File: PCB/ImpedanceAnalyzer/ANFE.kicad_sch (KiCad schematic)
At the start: 61 parts, among them U1 LTC2311, U10 OPA350, U11 OPA350, U2 LTC2311, U3 REF02Z, U4 LD1117S25-TR, U5 LD1117S50-TR, U7 LT1819, U9 OPA350

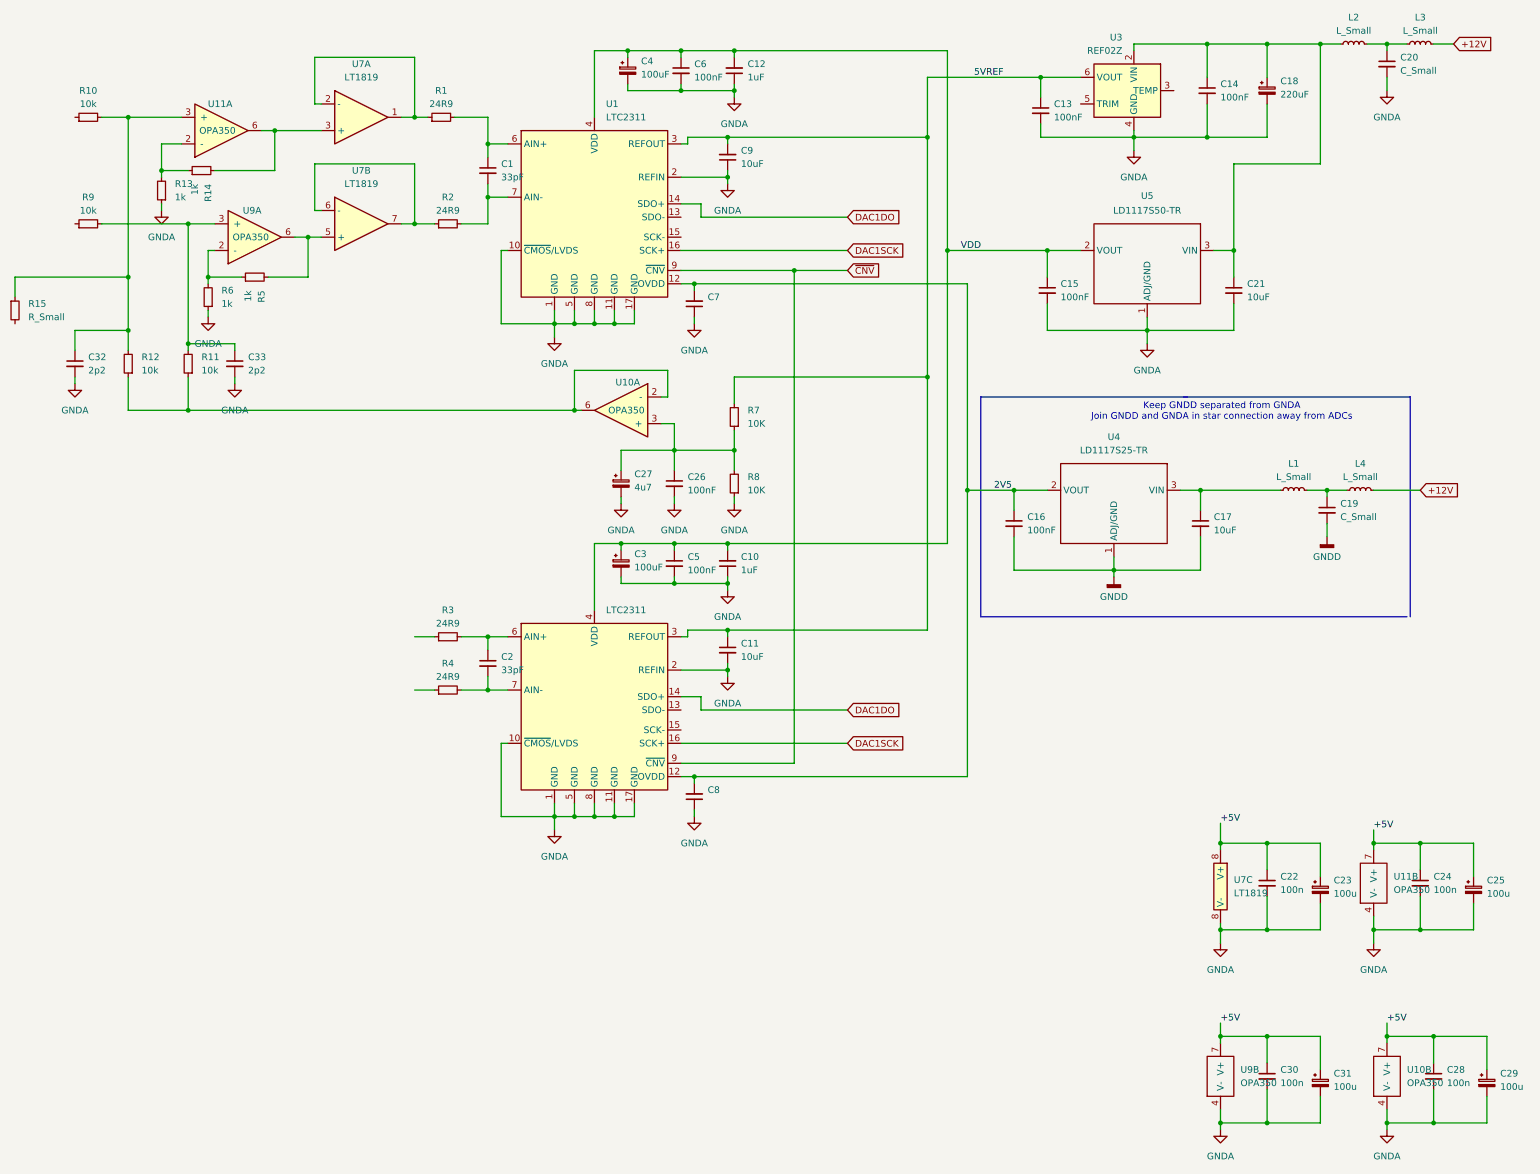
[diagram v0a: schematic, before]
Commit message: filter work
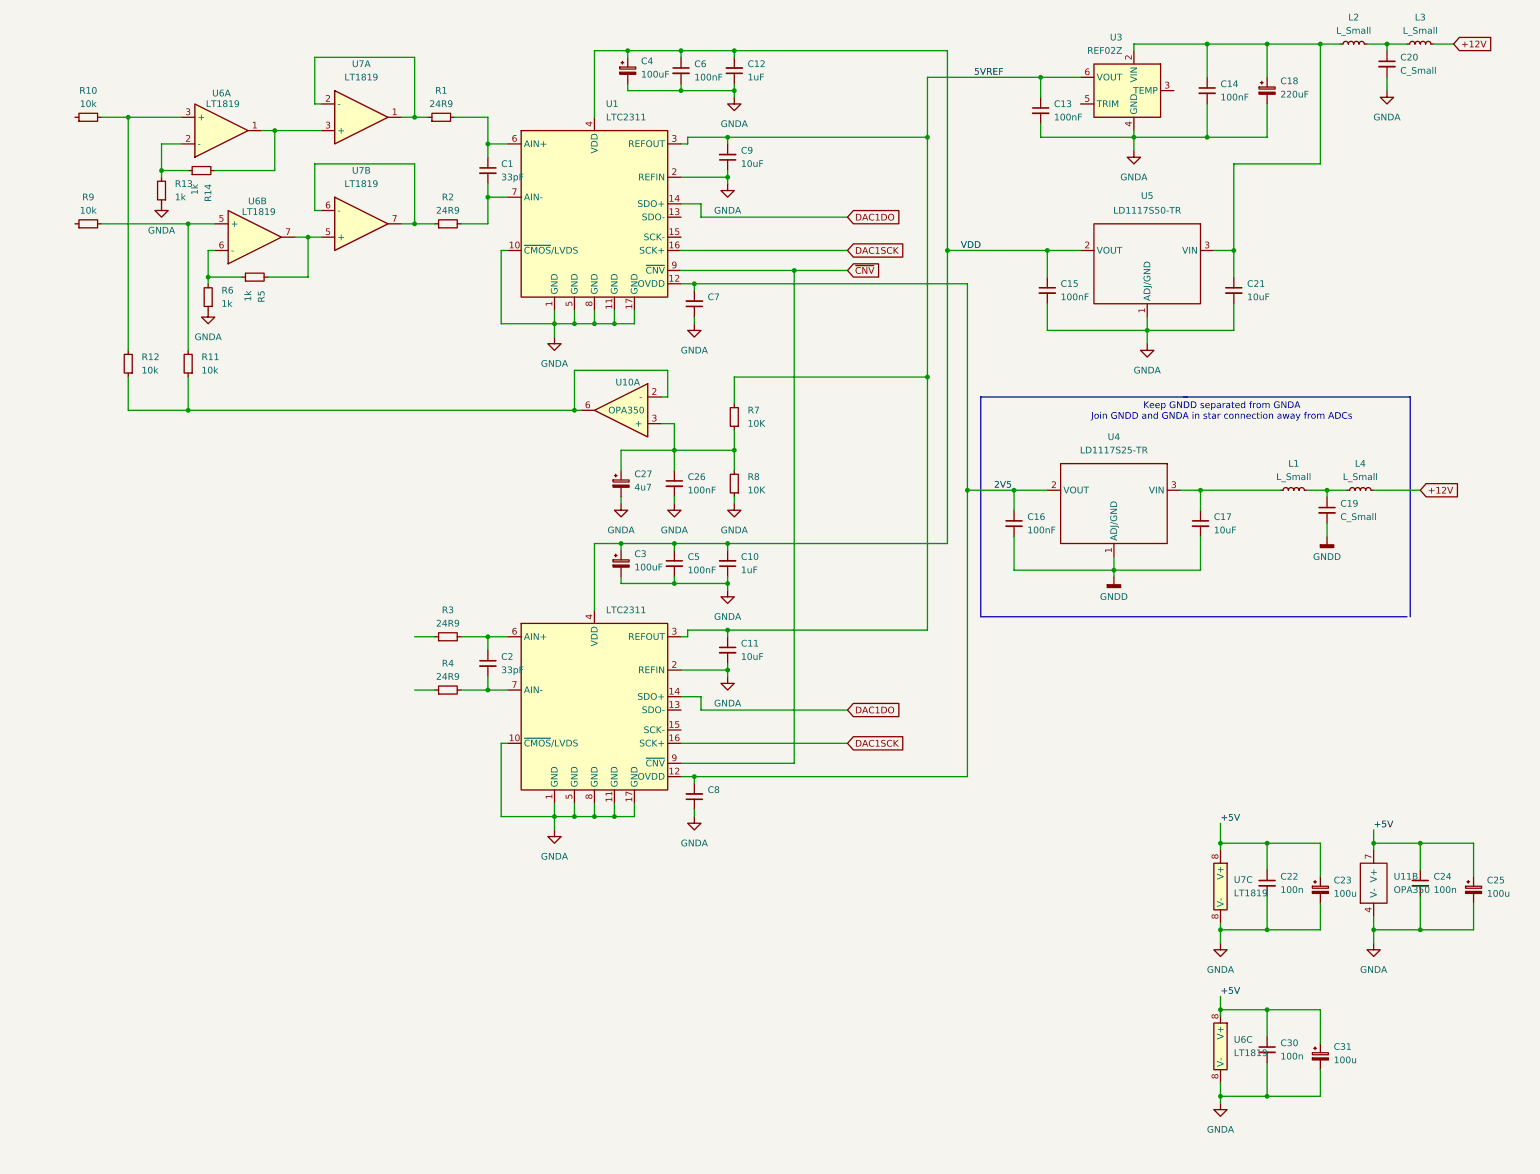
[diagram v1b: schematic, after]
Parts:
- removed C28: 100n, symbol Device:C_Small
- removed C29: 100u, symbol Device:C_Polarized_Small
- removed C32, C33: 2p2, symbol Device:C_Small
- removed R15: R_Small, symbol Device:R_Small
- removed unit 2 of U10
- removed unit 1 of U11
- removed U9: OPA350, symbol JRIX Op Amp:OPA350
- added U6: LT1819, symbol JRIX Op Amp:LT1819
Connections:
- net +5V: now also U6.8 (V-)
- net GNDA: now also U6.8 (V-)
- net at R5.1, R6.2: now also U6.6 (-)
- net at R5.2, U7.5 (+): now also U6.7
- net at R11.2, R9.2: now also U6.5 (+)
- net at R10.2, R12.2: now also U6.3 (+)
- net at R14.2, U7.3 (+): now also U6.1
- net at R13.2, R14.1: now also U6.2 (-)
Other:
- moved on the sheet: C30, C31
